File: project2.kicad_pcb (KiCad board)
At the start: 2 copper layers, 30 x 25 mm, 28 parts, among them J1 USB_C_Receptacle_PowerOnly_6P, J2 Conn_01x01_Socket, J3 Conn_01x01_Socket, J4 Conn_01x01_Socket, J5 Conn_01x01_Socket, Q1 FS8205A, Q2 DW01A, SW1 SW_Nidec_CAS-120A1, U1 TP4056-42-ESOP8, U2 MT3608

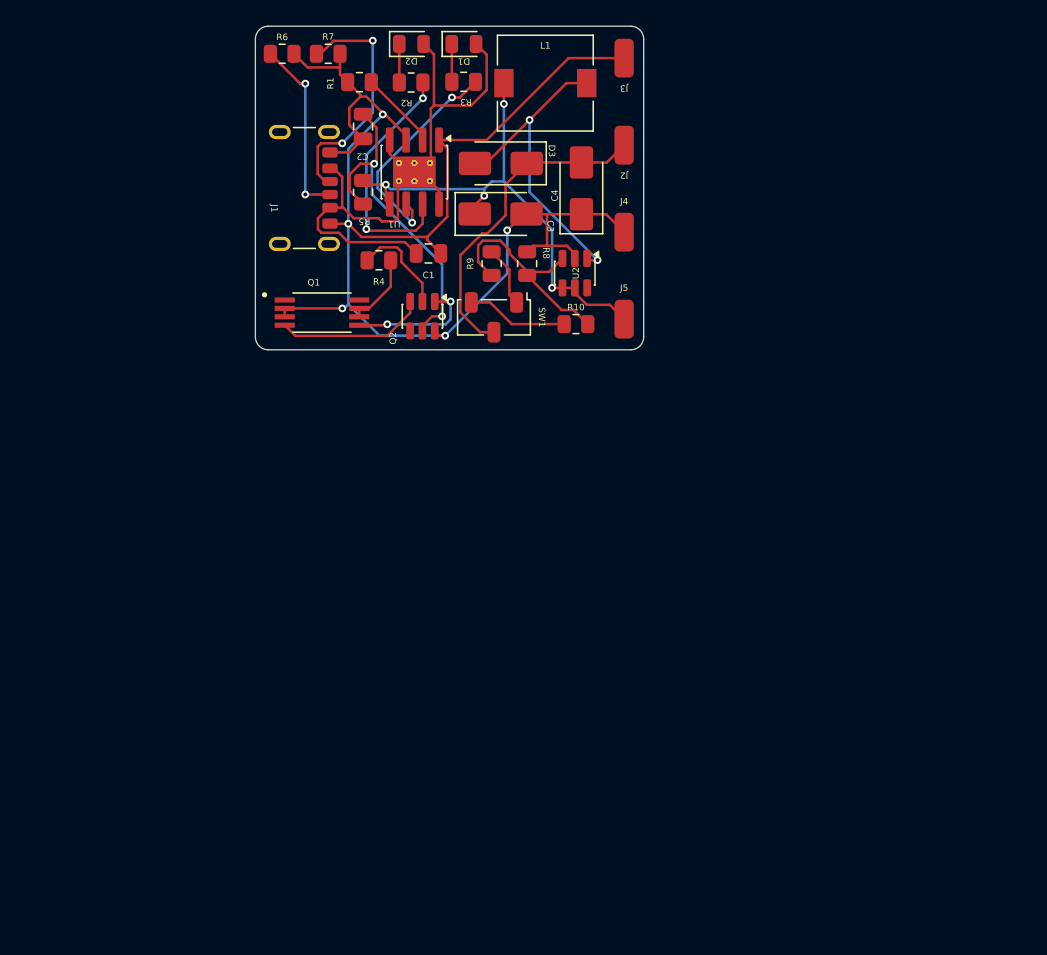
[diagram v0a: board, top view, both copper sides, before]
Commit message: Project Compleated v1.2
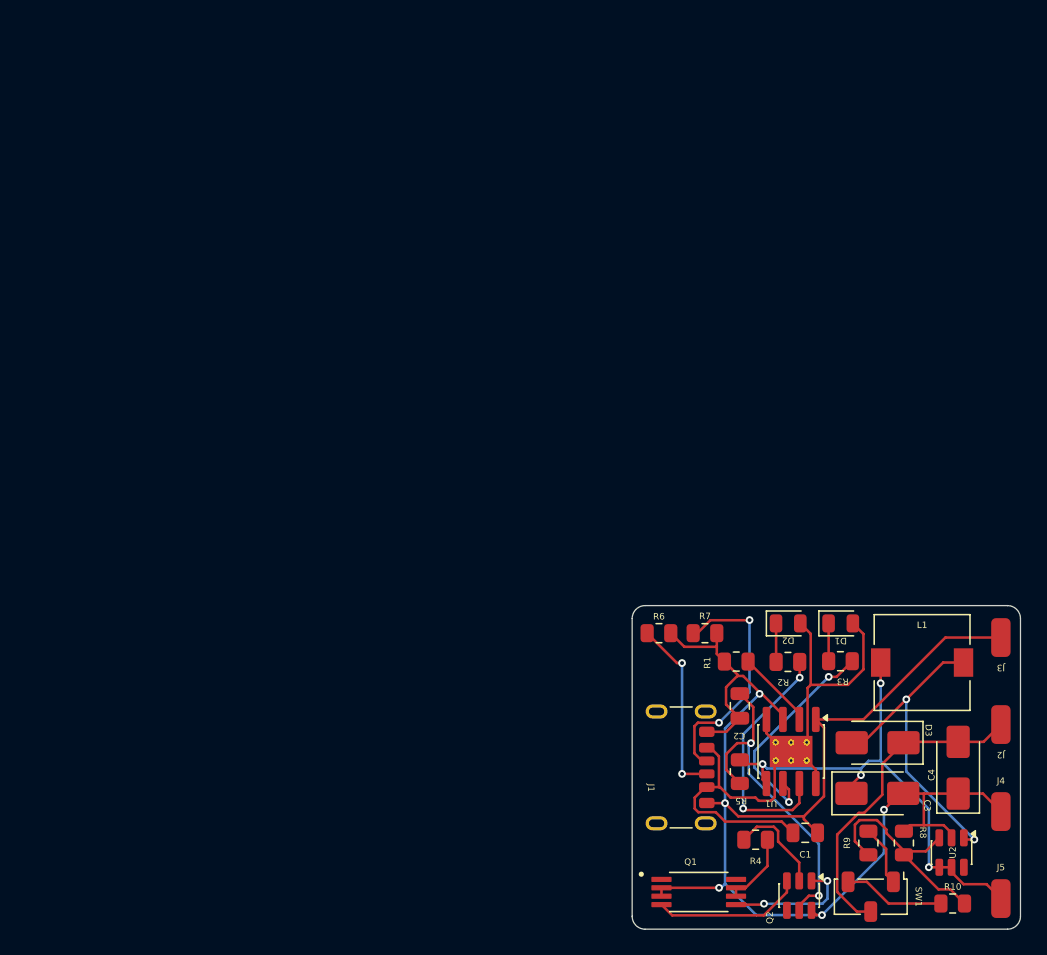
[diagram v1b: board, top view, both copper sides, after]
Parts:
- moved C1 53.4 mm to (234.8, 152.7)
- moved C3 53.4 mm to (240.3, 149.6)
- moved C4 53.4 mm to (246.6, 147.7)
- moved D1 53.4 mm to (237.5, 136.5)
- moved D2 53.4 mm to (233.5, 136.5)
- moved D3 53.4 mm to (240.4, 145.7)
- moved J1 53.4 mm to (224.1, 147.6)
- moved Q1 53.4 mm to (226.5, 157.3)
- moved R2 53.4 mm to (233.4, 139.5)
- moved R4 53.4 mm to (230.9, 153.2)
- moved R6 53.4 mm to (223.5, 137.3)
- moved R7 53.4 mm to (227.0, 137.3)
- moved U1 53.4 mm to (233.7, 146.4)
- moved U2 53.4 mm to (246.1, 154.2)
- moved C2 53.4 mm to (229.7, 142.9)
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
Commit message: PROJECT COMPLEATED
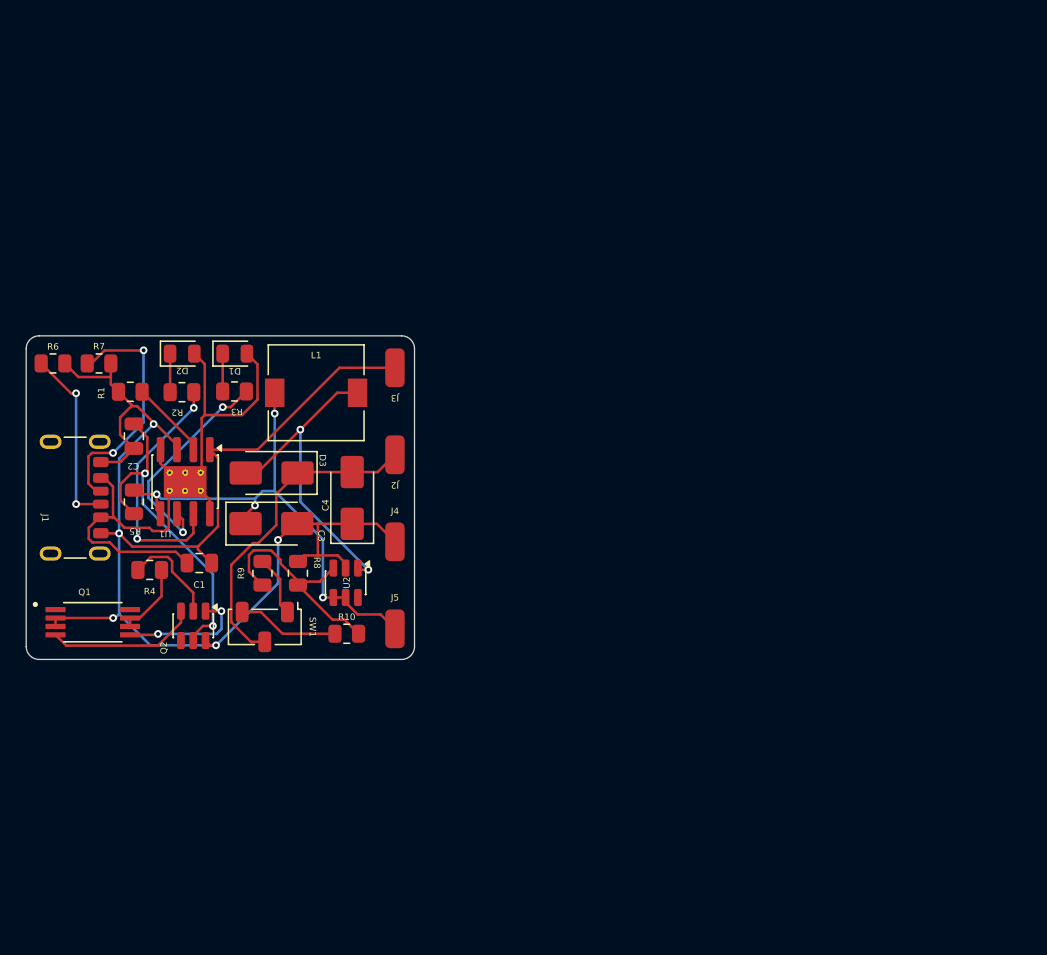
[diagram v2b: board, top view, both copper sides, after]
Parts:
- moved C1 51.2 mm to (188.0, 131.8)
- moved J3 51.2 mm to (203.1, 116.8)
- moved R2 51.2 mm to (186.6, 118.6)
- moved J2 51.2 mm to (203.1, 123.5)
- moved J4 51.2 mm to (203.1, 130.2)
- moved J5 51.2 mm to (203.1, 136.9)
- moved R9 51.2 mm to (192.8, 132.6)
- moved C3 51.2 mm to (193.5, 128.8)
- moved D3 51.2 mm to (193.5, 124.9)
- moved J1 51.2 mm to (177.3, 126.8)
- moved Q1 51.2 mm to (179.7, 136.4)
- moved R4 51.2 mm to (184.1, 132.4)
- moved U2 51.2 mm to (199.3, 133.4)
- moved C2 51.2 mm to (182.9, 122.0)
- moved C4 51.2 mm to (199.8, 126.8)
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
